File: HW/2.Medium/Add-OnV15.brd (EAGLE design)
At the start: 28.1 x 17.6 mm, 10 parts, among them X1 1501_03

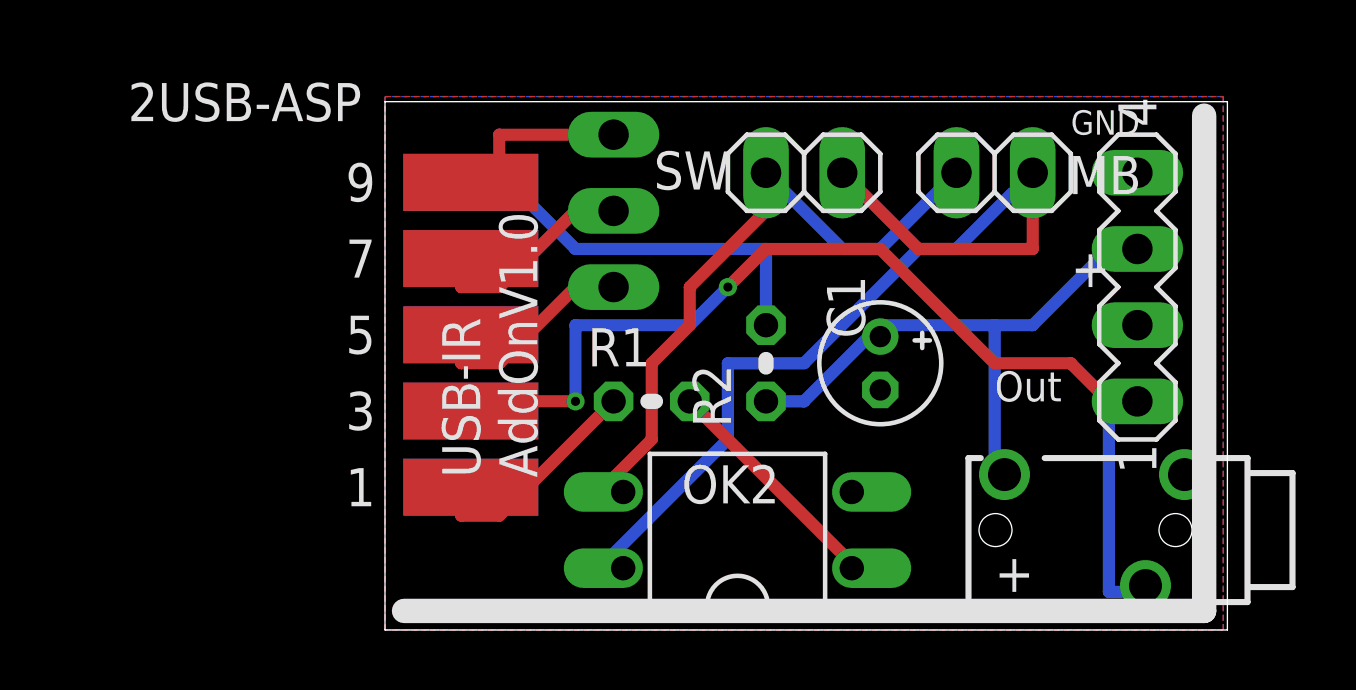
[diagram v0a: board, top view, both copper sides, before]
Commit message: Mini V1.1
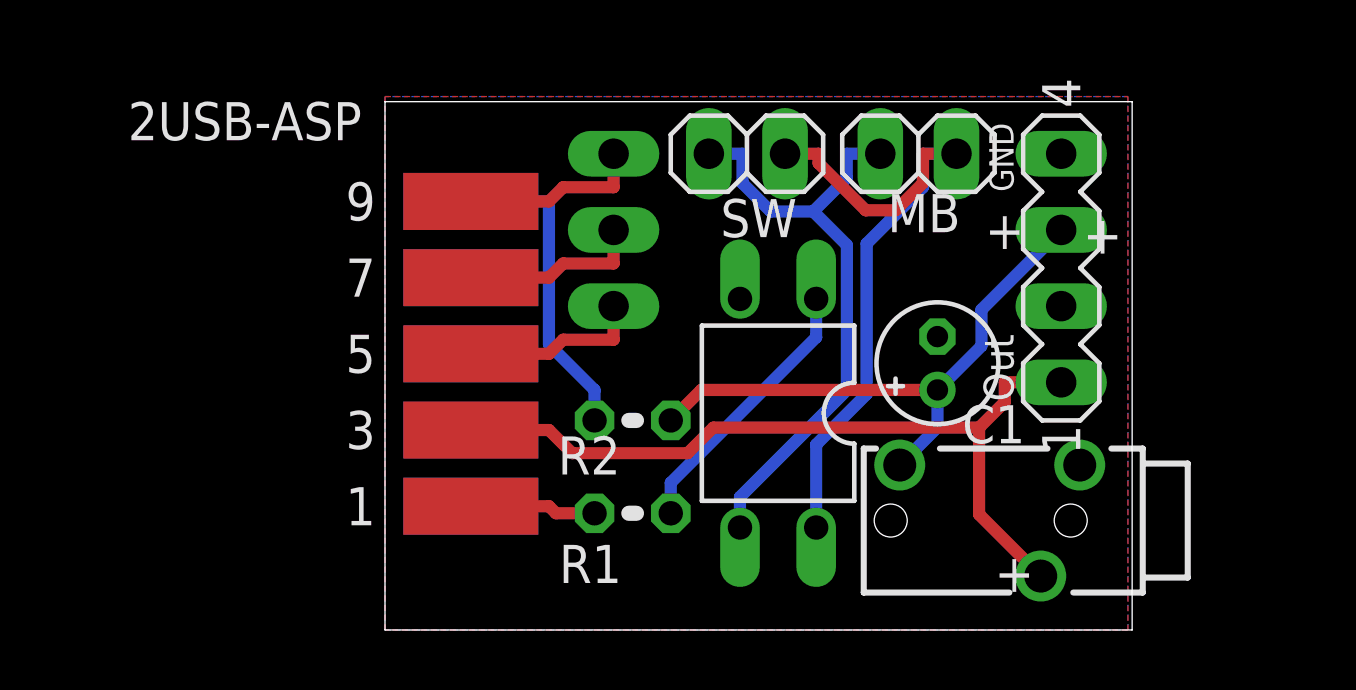
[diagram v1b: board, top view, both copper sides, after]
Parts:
- moved R2 4.84 mm to (8.26, 6.99), turned to 180 degrees
- moved OK2 4.12 mm to (13.1, 7.22), turned to 180 degrees
- moved R1 3.78 mm to (8.26, 3.89)
- moved X1 3.51 mm to (22.9, 3.65)
- moved MB 2.62 mm to (17.8, 15.9)
- moved SV1 2.62 mm to (22.5, 12.1)
- moved SW 2.01 mm to (12.1, 15.9)
- moved C1 1.90 mm to (18.4, 8.89), turned to 90 degrees
- moved 2USB-ASP 0.63 mm to (2.86, 9.21)
- moved FREI 0.63 mm to (7.62, 13.3)
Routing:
- net SCK: track 36.8 -> 27.2 mm, vias 2 -> 0
- net N$3: track 31.2 -> 23.1 mm
- net MISO: track 8.38 -> 4.22 mm
- net VCC: track 13.5 -> 10.5 mm
- net RST: track 7.85 -> 6.07 mm
- net NC: track 7.85 -> 6.07 mm
- net N$2: track 7.76 -> 9.15 mm
- net N$1: track 20.7 -> 19.4 mm
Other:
- board size 28.1 x 17.6 mm -> 24.9 x 17.6 mm
- board text added: "USB-IR Med V1.1"
- board text added: "www.neuby.de"
- board text removed: "USB-IR AddOnV1.0"
